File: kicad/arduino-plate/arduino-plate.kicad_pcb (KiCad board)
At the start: 2 copper layers, 49.5 x 62.2 mm, 10 parts

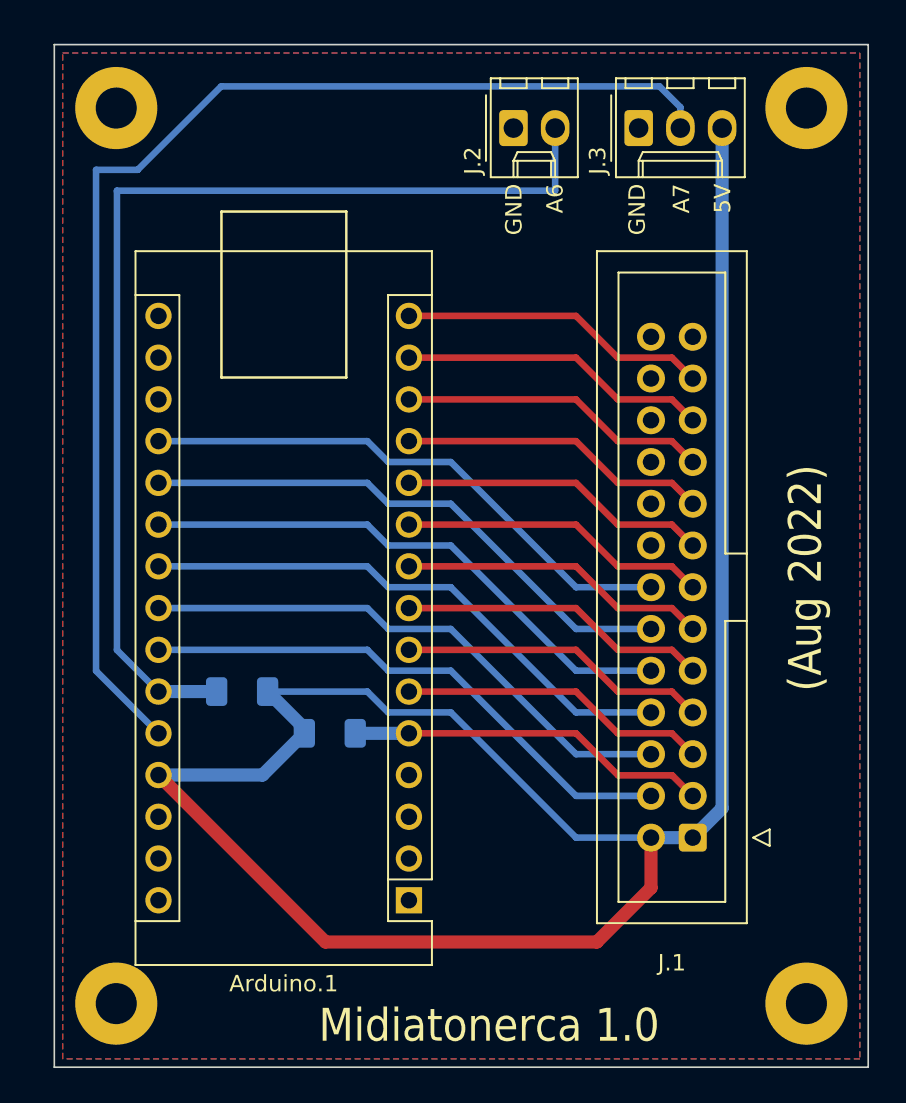
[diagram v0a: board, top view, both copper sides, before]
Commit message: Updates to arduino
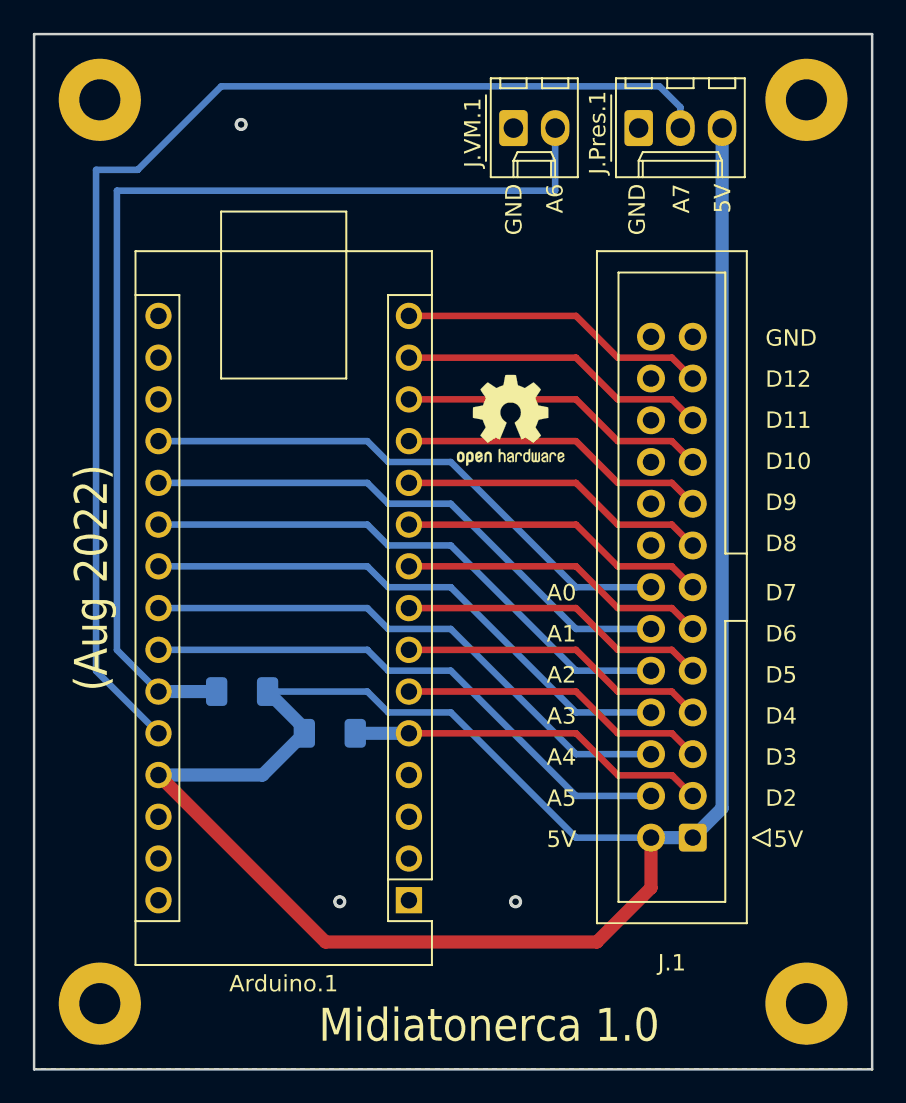
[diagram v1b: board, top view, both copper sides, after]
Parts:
- added REF**: OSHW-Logo2_7.3x6mm_SilkScreen, Symbol:OSHW-Logo2_7.3x6mm_SilkScreen, F.Cu at (90.0, 63.5)
- moved ? 1.12 mm to (65.0, 44.0)
- moved ? 1.00 mm to (65.0, 99.0)
- moved ? 0.50 mm to (108.0, 44.0)
- renumbered J.3 to J.Pres.1, J.2 to J.VM.1
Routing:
- net GND: vias 0 -> 3
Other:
- board size 49.5 x 62.2 mm -> 51 x 63 mm
- board text added: "A0"
- board text added: "A1"
- board text added: "A2"
- board text added: "A3"
- board text added: "A4"
- board text added: "A5"
- board text added: "D10"
- board text added: "D11"
- board text added: "D12"
- board text added: "D2"
- board text added: "D3"
- board text added: "D4"
- board text added: "D5"
- board text added: "D6"
- board text added: "D7"
- board text added: "D8"
- board text added: "D9"
